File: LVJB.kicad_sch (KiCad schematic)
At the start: 18 parts, among them J1 Section H1, J10 Section F, J11 Section E1, J12 Section E2, J13 Section E3, J14 Section T1A, J2 Section A1, J3 Section A2, J4 Section A3, J5 Section A4, J6 Section M, J7 Section B1, J8 Section B2, J9 Section K

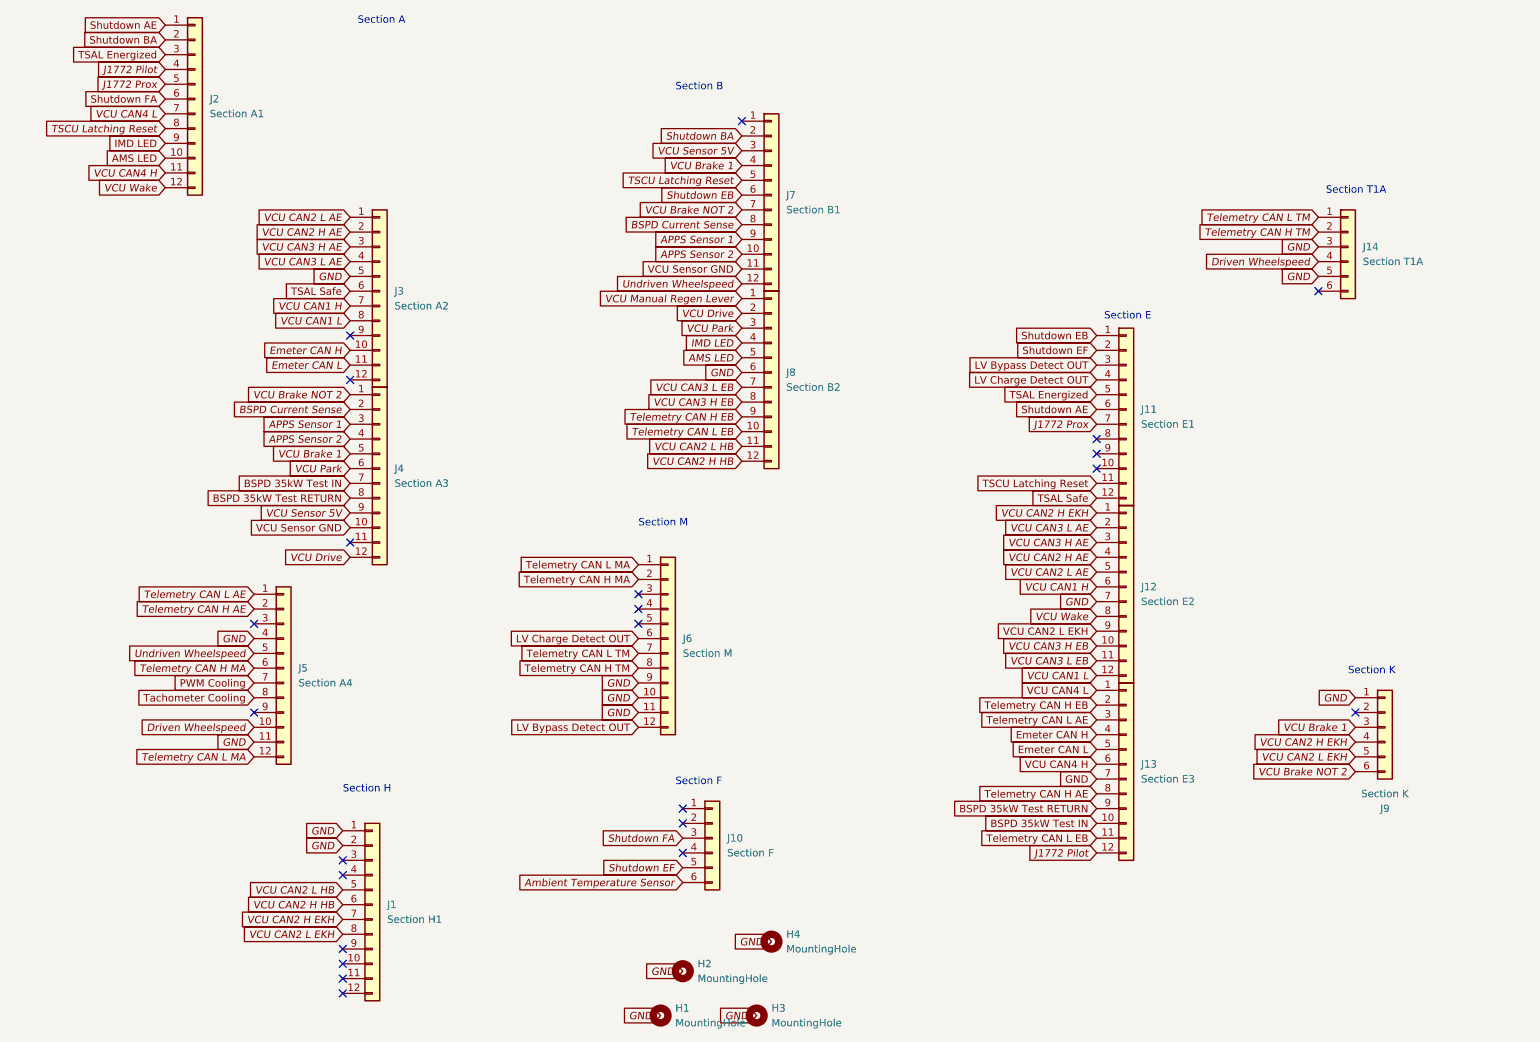
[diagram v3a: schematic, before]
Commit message: Added the 24V pin locations and fixed other issues
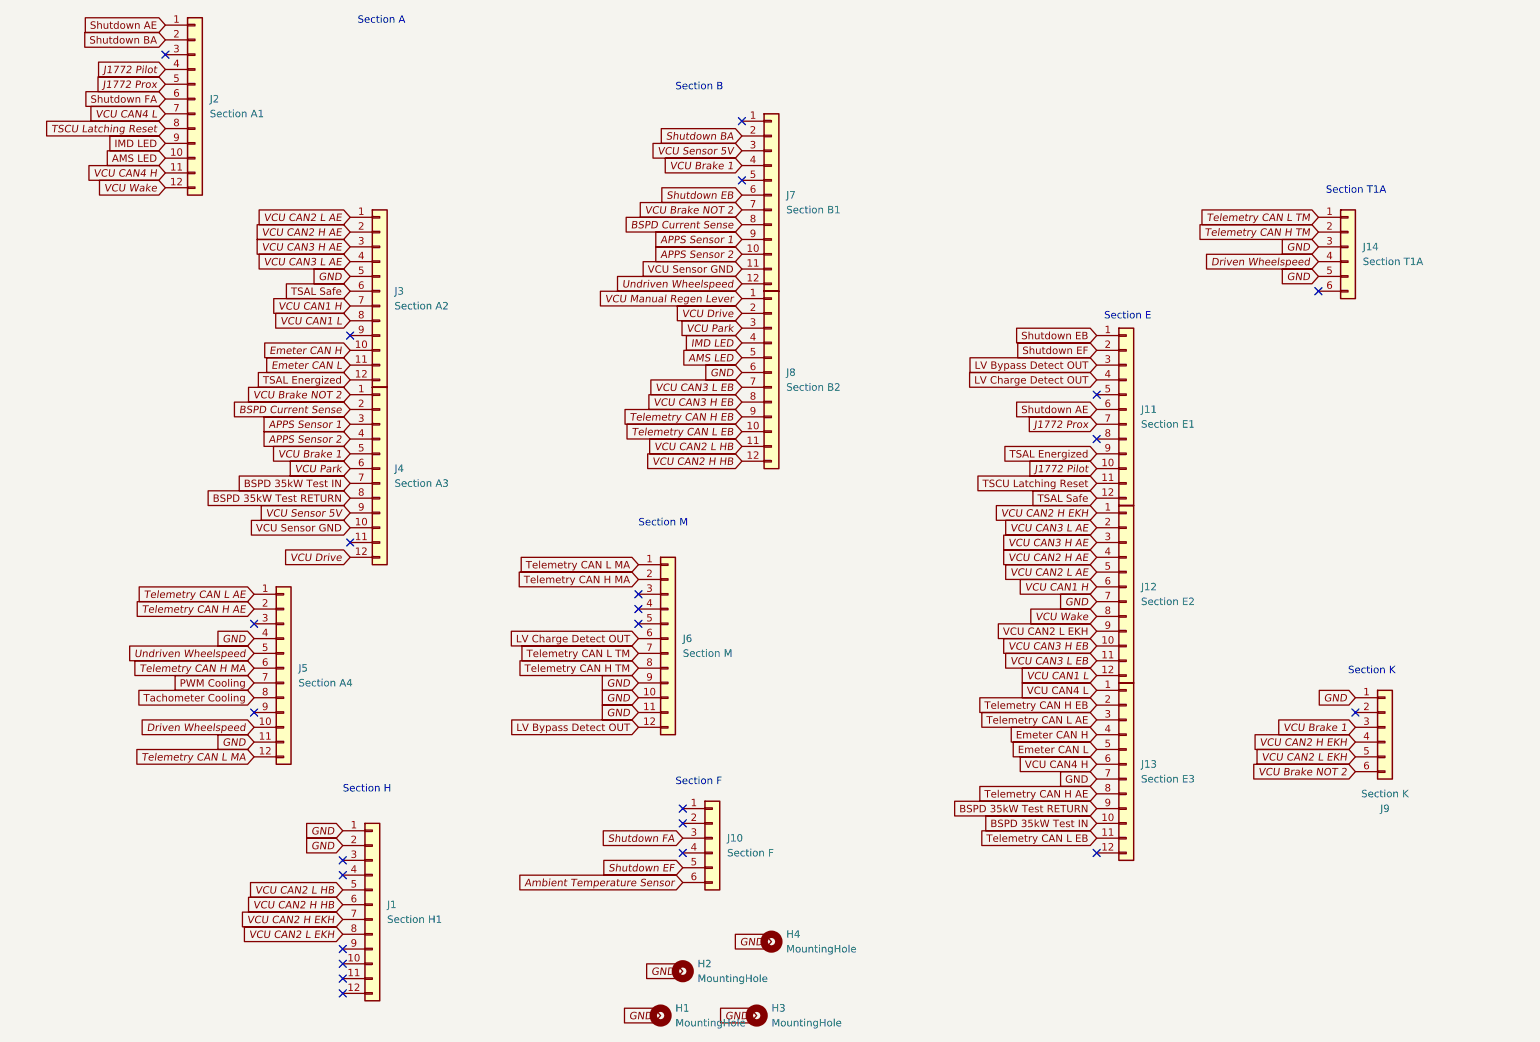
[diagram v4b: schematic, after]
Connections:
- net J1772 Pilot: now also J11.10 (Pin_10); no longer J13.12 (Pin_12)
- net TSAL Energized: now also J11.9 (Pin_9), J3.12 (Pin_12); no longer J11.5 (Pin_5), J2.3 (Pin_3)
- net TSCU Latching Reset: no longer J7.5 (Pin_5)
- no-connect marks 23 -> 24
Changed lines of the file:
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@@
   (no_connect (at 44.45 137.16))
   (no_connect (at 233.68 137.16))
+  (no_connect (at 128.27 45.72))
+  (no_connect (at 29.21 24.13))
+  (no_connect (at 189.23 82.55))
+  (no_connect (at 189.23 161.29))
   (no_connect (at 44.45 121.92))
-  (no_connect (at 189.23 95.25))
-  (no_connect (at 189.23 92.71))
   (no_connect (at 189.23 90.17))
   (no_connect (at 128.27 35.56))
@@
   (no_connect (at 110.49 119.38))
   (no_connect (at 110.49 121.92))
-  (no_connect (at 60.96 80.01))
   (no_connect (at 60.96 72.39))
   (no_connect (at 59.69 162.56))
@@
     )
   )
-  (global_label "TSAL Energized" (shape input) (at 189.23 82.55 180) (fields_autoplaced)
-    (effects (font (size 1.27 1.27)) (justify right))
-    (property "Intersheet References" "${INTERSHEET_REFS}" (id 0) (at 172.3631 82.4706 0)
-      (effects (font (size 1.27 1.27)) (justify right) hide)
-    )
-  )
   (global_label "Shutdown EF" (shape input) (at 118.11 163.83 180) (fields_autoplaced)
     (effects (font (size 1.27 1.27) italic) (justify right))
@@
     )
   )
-  (global_label "TSAL Energized" (shape input) (at 29.21 24.13 180) (fields_autoplaced)
-    (effects (font (size 1.27 1.27)) (justify right))
-    (property "Intersheet References" "${INTERSHEET_REFS}" (id 0) (at 12.3431 24.0506 0)
-      (effects (font (size 1.27 1.27)) (justify right) hide)
-    )
-  )
   (global_label "BSPD Current Sense" (shape input) (at 60.96 85.09 180) (fields_autoplaced)
     (effects (font (size 1.27 1.27) italic) (justify right))
@@
     )
   )
+  (global_label "J1772 Pilot" (shape input) (at 189.23 95.25 180) (fields_autoplaced)
+    (effects (font (size 1.27 1.27) italic) (justify right))
+    (property "Intersheet References" "${INTERSHEET_REFS}" (id 0) (at 175.3732 95.1706 0)
+      (effects (font (size 1.27 1.27) italic) (justify right) hide)
+    )
+  )
   (global_label "GND" (shape input) (at 189.23 148.59 180) (fields_autoplaced)
     (effects (font (size 1.27 1.27)) (justify right))
@@
     )
   )
+  (global_label "TSAL Energized" (shape input) (at 60.96 80.01 180) (fields_autoplaced)
+    (effects (font (size 1.27 1.27)) (justify right))
+    (property "Intersheet References" "${INTERSHEET_REFS}" (id 0) (at 44.0931 79.9306 0)
+      (effects (font (size 1.27 1.27)) (justify right) hide)
+    )
+  )
   (global_label "GND" (shape input) (at 44.45 124.46 180) (fields_autoplaced)
     (effects (font (size 1.27 1.27) italic) (justify right))
@@
     )
   )
-  (global_label "J1772 Pilot" (shape input) (at 189.23 161.29 180) (fields_autoplaced)
-    (effects (font (size 1.27 1.27) italic) (justify right))
-    (property "Intersheet References" "${INTERSHEET_REFS}" (id 0) (at 175.3732 161.2106 0)
-      (effects (font (size 1.27 1.27) italic) (justify right) hide)
-    )
-  )
   (global_label "VCU CAN1 L" (shape input) (at 60.96 69.85 180) (fields_autoplaced)
     (effects (font (size 1.27 1.27) italic) (justify right))
@@
     )
   )
+  (global_label "TSAL Energized" (shape input) (at 189.23 92.71 180) (fields_autoplaced)
+    (effects (font (size 1.27 1.27)) (justify right))
+    (property "Intersheet References" "${INTERSHEET_REFS}" (id 0) (at 172.3631 92.6306 0)
+      (effects (font (size 1.27 1.27)) (justify right) hide)
+    )
+  )
   (global_label "VCU CAN2 H AE" (shape input) (at 60.96 54.61 180) (fields_autoplaced)
     (effects (font (size 1.27 1.27) italic) (justify right))
@@
       (effects (font (size 1.27 1.27) italic) (justify right) hide)
     )
-  )
-  (global_label "TSCU Latching Reset" (shape input) (at 128.27 45.72 180) (fields_autoplaced)
-    (effects (font (size 1.27 1.27) italic) (justify right))
-    (property "Intersheet References" "${INTERSHEET_REFS}" (id 0) (at 105.6442 45.6406 0)
-      (effects (font (size 1.27 1.27) italic) (justify right) hide)
-    )
